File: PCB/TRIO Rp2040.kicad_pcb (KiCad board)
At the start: 2 copper layers, 22.5 x 25.3 mm, 27 parts, among them J1 USB_C_Receptacle_USB2.0_16P, J2 Conn_01x02_Pin, J3 Conn_01x02_Pin, J5 Conn_01x07_Pin, J6 Conn_01x07_Pin, J7 Conn_01x07_Pin, SW1 SW_Push, U1 RP2040, U2 MCP1700x-330xxTT, U4 W25Q16JVUXIQ TR, Y1 12 MHz

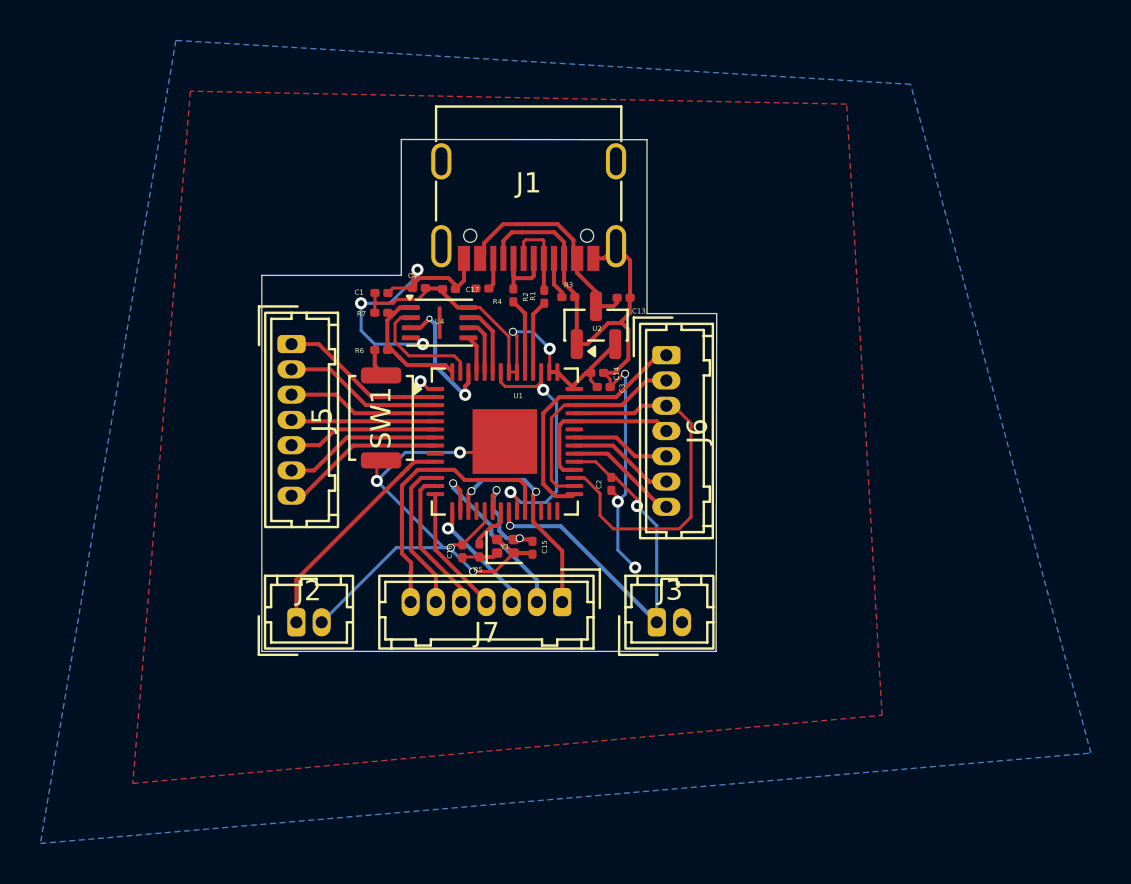
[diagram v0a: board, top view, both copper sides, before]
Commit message: Add files via upload
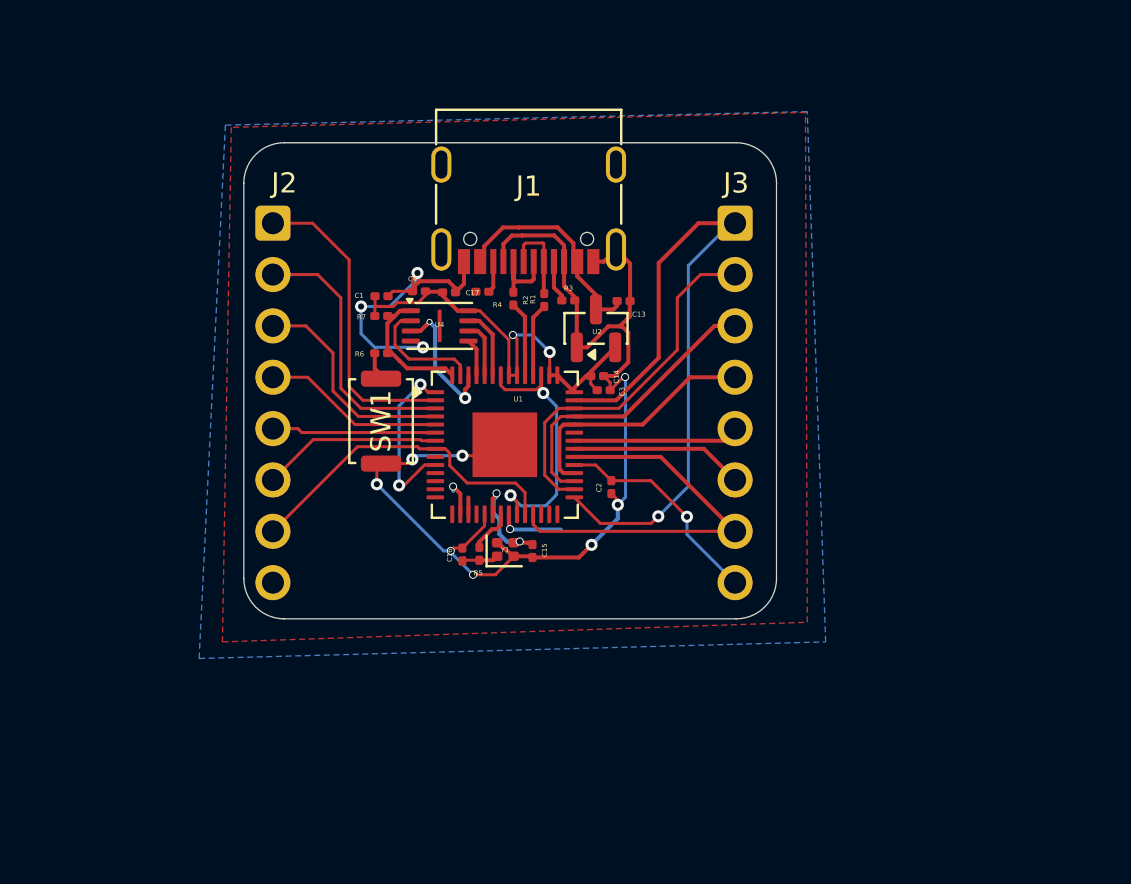
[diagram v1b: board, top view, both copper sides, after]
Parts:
- removed J5, J6, J7: Conn_01x07_Pin, Connector_Hirose:Hirose_DF13-07P-1.25DSA_1x07_P1.25mm_Vertical
- J2, J3: value Conn_01x02_Pin -> Conn_01x08_Pin; footprint Connector_Hirose:Hirose_DF13-02P-1.25DSA_1x02_P1.25mm_Vertical -> Connector_Molex:Molex_SL_171971-0008_1x08_P2.54mm_Vertical
- moved J3 20.1 mm to (129.5, 58.4), turned to -90 degrees
- moved J2 19.8 mm to (106.7, 58.4), turned to -90 degrees
- moved C14 0.16 mm to (122.7, 66.0)
- moved C15 0.16 mm to (119.5, 74.6)
- moved C3 0.16 mm to (123.0, 66.7)
- moved C1 0.16 mm to (112.0, 62.0)
- moved C13 0.16 mm to (124.0, 62.3)
- moved C17 0.16 mm to (115.4, 61.8)
- moved R3 0.16 mm to (121.3, 62.2)
- moved R4 0.16 mm to (117.0, 61.8)
- moved U2 0.16 mm to (122.7, 63.6)
- moved C16 0.16 mm to (116.0, 74.8)
- moved C2 0.16 mm to (123.4, 71.5)
- moved C4 0.16 mm to (113.9, 61.8)
- moved J1 0.16 mm to (119.3, 56.6)
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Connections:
- J2 pad 1: 3.3V -> GPIO0
- J2 pad 2: GND -> GPIO1
- J3 pad 1: 3.3V -> GPIO18
- J3 pad 2: GND -> GPIO19
- U1 pad 11: GPIO8 -> unconnected-(U1-GPIO8-Pad11)
- U1 pad 12: GPIO9 -> unconnected-(U1-GPIO9-Pad12)
- U1 pad 13: GPIO10 -> unconnected-(U1-GPIO10-Pad13)
- U1 pad 14: GPIO11 -> unconnected-(U1-GPIO11-Pad14)
- U1 pad 15: GPIO12 -> unconnected-(U1-GPIO12-Pad15)
- U1 pad 16: GPIO13 -> unconnected-(U1-GPIO13-Pad16)
- U1 pad 17: GPIO14 -> unconnected-(U1-GPIO14-Pad17)
- U1 pad 24: GPIO8 -> GPIO6
- U1 pad 25: GPIO14 -> GPIO22
- U1 pad 26: RUN -> unconnected-(U1-RUN-Pad26)
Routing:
- net GPIO18: track 12.6 -> 35.4 mm, vias 0 -> 1
- net GPIO22: track 5.64 -> 20.1 mm
- net GPIO8: track 14.2 -> 0.00 mm
- net GPIO14: track 10.8 -> 0.00 mm, vias 2 -> 0
- net 3.3V: track 55.0 -> 45.0 mm, vias 5 -> 6
- net GPIO13: track 9.12 -> 0.00 mm, vias 1 -> 0
- net GPIO6: track 8.14 -> 16.6 mm
- net GPIO9: track 7.79 -> 0.00 mm
- net GPIO19: track 10.8 -> 18.3 mm
- net GPIO10: track 7.19 -> 0.00 mm
- net GPIO0: track 8.20 -> 15.3 mm
- net GND: track 79.1 -> 72.2 mm, vias 10 -> 11
- net GPIO11: track 6.39 -> 0.00 mm
- net GPIO12: track 5.96 -> 0.00 mm, vias 1 -> 0
- net GPIO1: track 7.85 -> 13.4 mm
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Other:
- board size 22.5 x 25.3 mm -> 26.4 x 23.5 mm
